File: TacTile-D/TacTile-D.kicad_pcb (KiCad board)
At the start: 2 copper layers, 59.9 x 59.9 mm, 19 parts, among them J1 Conn_01x06, J2 Conn_01x06, J3 Conn_01x06, J4 Conn_01x06, J5 Conn_01x04, J6 Conn_01x05, J7 Conn_01x02, J8 Conn_01x02, U1 74LVC2G08, U10 74LVC1G373, U11 74AUC1G74, U2 74LVC2G04, U3 74HC595, U4 74HC590, U5 74LVC2G00, U6 74LS74, U7 74LVC2G32, U8 74LVC1G18, U9 74LVC2G04

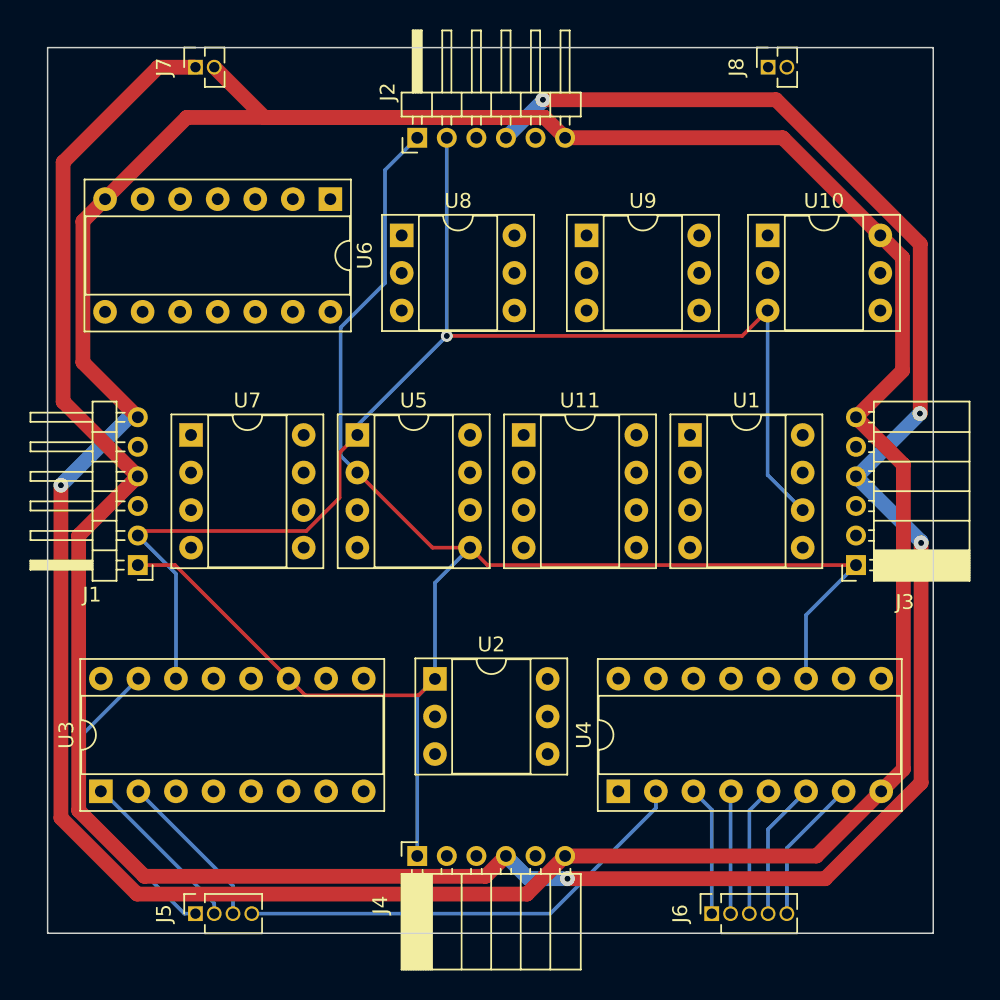
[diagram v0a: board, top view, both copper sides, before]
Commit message: Finished board D routing
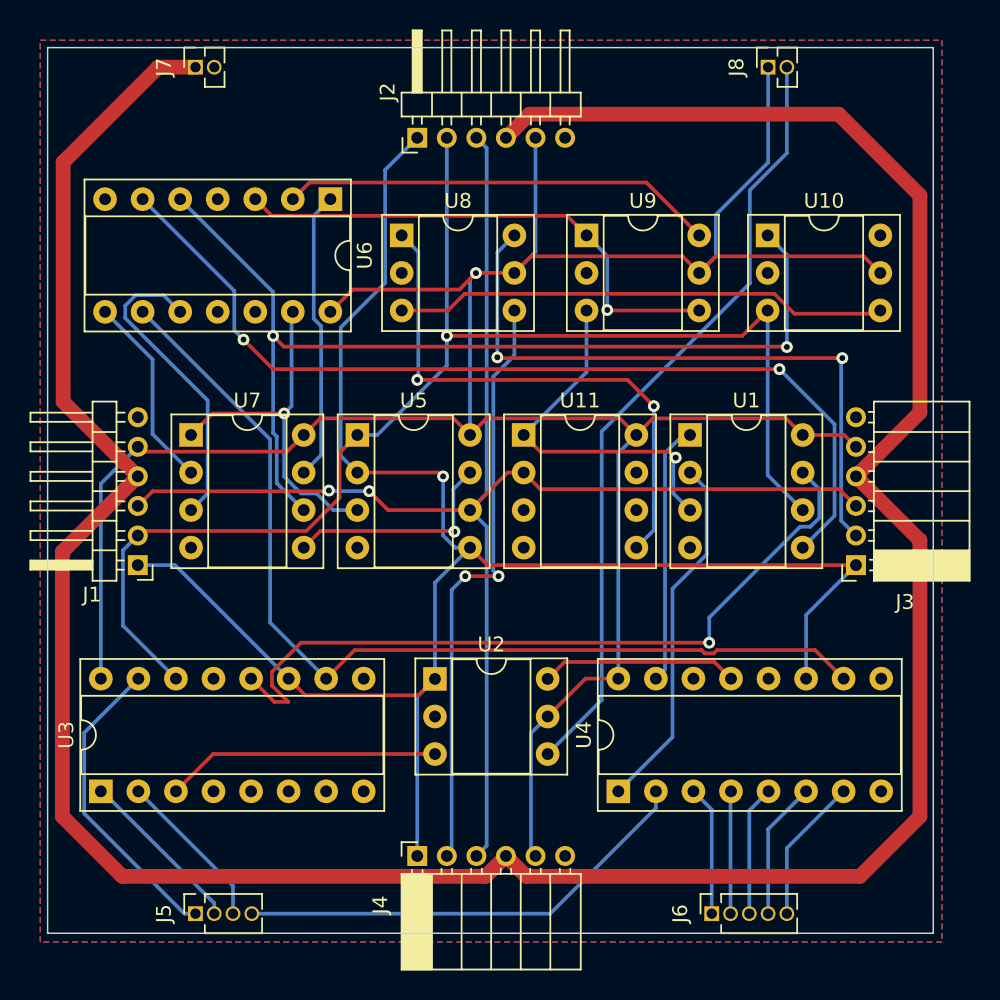
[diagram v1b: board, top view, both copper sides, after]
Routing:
- net GND: track 230.3 -> 0.00 mm, vias 1 -> 0
- net VCC: track 0.00 -> 178.7 mm, vias 0 -> 1
- net SS: track 0.00 -> 101.6 mm, vias 0 -> 2
- net Net-(U10-LE): track 0.00 -> 67.6 mm, vias 0 -> 2
- net SEN: track 0.00 -> 66.7 mm
- net Net-(U6A-~{Q}): track 0.00 -> 63.9 mm, vias 0 -> 2
- net LEN: track 0.00 -> 53.2 mm
- net Net-(U3-RCLK): track 0.00 -> 51.5 mm, vias 0 -> 1
- net MISO0: track 0.00 -> 44.5 mm, vias 0 -> 2
- net MISO1: track 0.00 -> 40.4 mm, vias 0 -> 2
- net Net-(U11-Q): track 0.00 -> 37.1 mm, vias 0 -> 2
- net Net-(U6A-C): track 0.00 -> 35.3 mm, vias 0 -> 1
- net Net-(U10-Q): track 0.00 -> 33.5 mm
- net Net-(U6A-D): track 0.00 -> 29.4 mm
- net Net-(U11-C): track 0.00 -> 25.2 mm, vias 0 -> 1
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- added copper zone on B.Cu, net GND
- added copper zone on F.Cu, net GND
